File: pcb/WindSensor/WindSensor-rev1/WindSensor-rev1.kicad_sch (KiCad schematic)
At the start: 14 parts, among them U1 Sensor_Wind, U2 Sensor_Wind, U3 Sensor_Wind, U4 LP5814DRLR

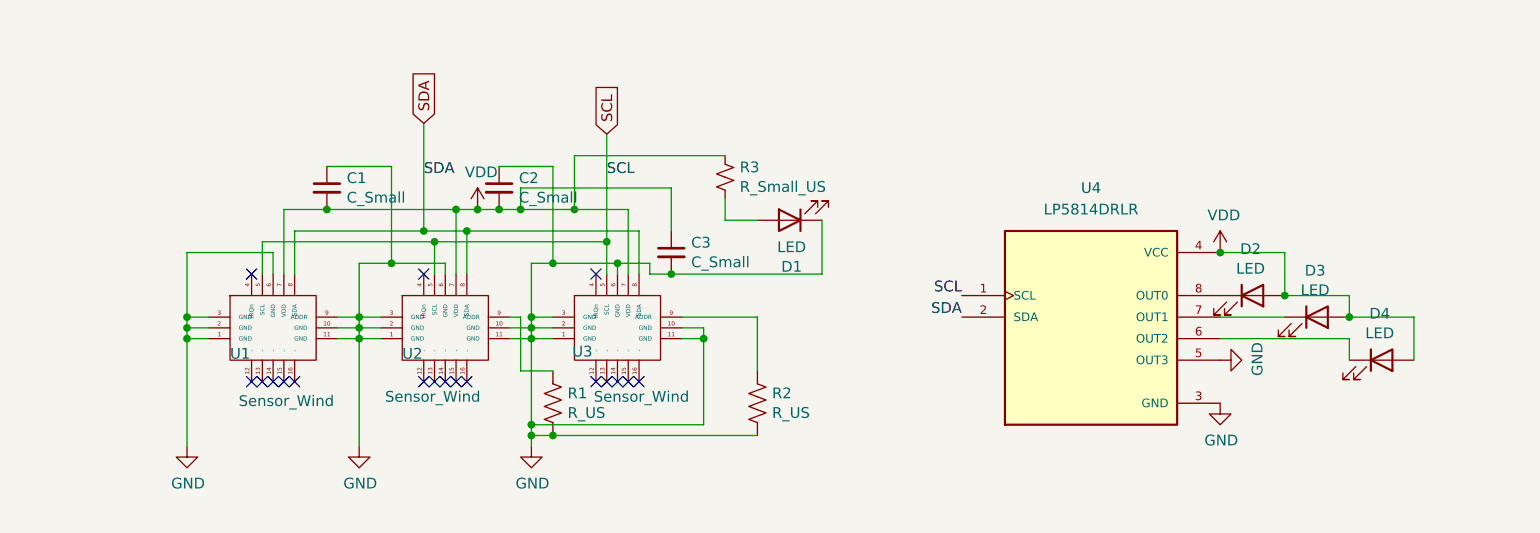
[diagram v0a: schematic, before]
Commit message: getting there
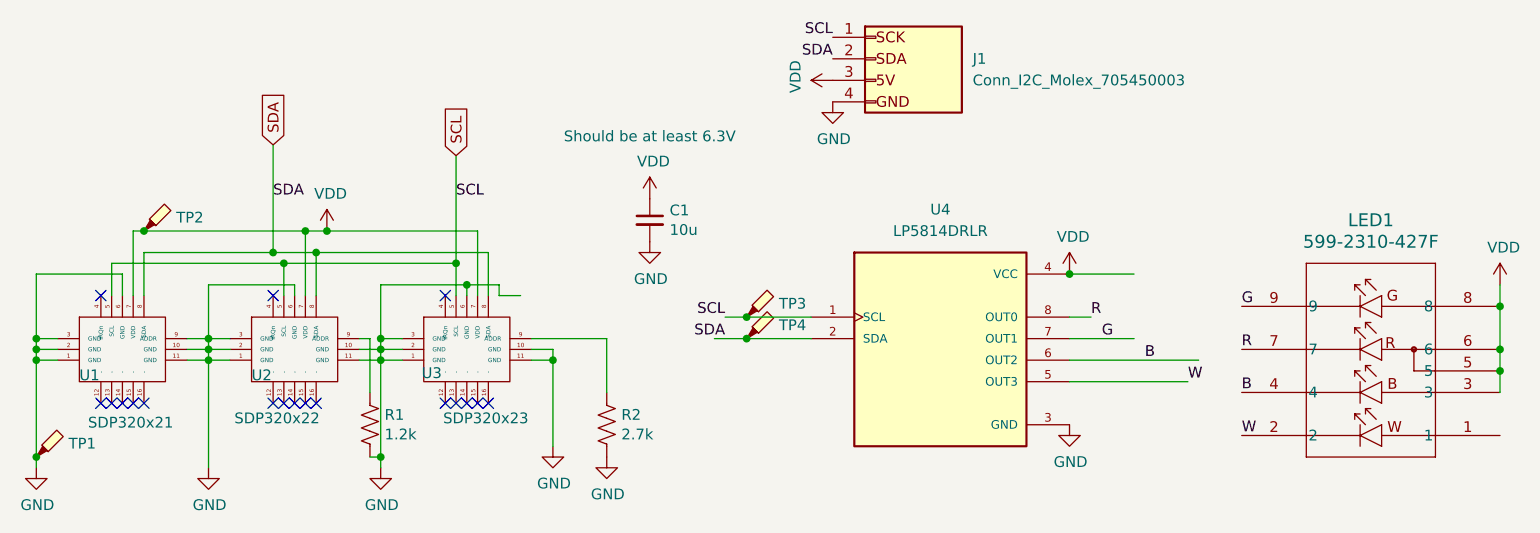
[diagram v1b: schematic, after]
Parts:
- removed C2, C3: C_Small, Capacitor_SMD:C_0201_0603Metric, symbol Device:C_Small
- removed D1, D2, D3, D4: LED, WindSensor:LED_3528, symbol Device:LED
- removed R3: R_Small_US, Resistor_SMD:R_0201_0603Metric, symbol Device:R_Small_US
- added J1: Conn_I2C_Molex_705450003, WindSensor:CONN_SD-74099-1000_04_MOL, symbol WindSensor:Conn_I2C_Molex_740990604
- added LED1: 599-2310-427F, WindSensor:599-2310_DIA, symbol WindSensor:599-2310-427F
- added TP1, TP2, TP3, TP4: TestPoint_Probe_autonamed, argo:TestPoint_scope_probe_autonamed, symbol argo:TestPoint_Probe_autonamed
- C1: value C_Small -> 10u; footprint Capacitor_SMD:C_0201_0603Metric -> Capacitor_SMD:C_0603_1608Metric_Pad1.08x0.95mm_HandSolder
- R1: value R_US -> 1.2k; footprint Resistor_SMD:R_0201_0603Metric -> Resistor_SMD:R_0603_1608Metric_Pad0.98x0.95mm_HandSolder
- R2: value R_US -> 2.7k; footprint Resistor_SMD:R_0201_0603Metric -> Resistor_SMD:R_0603_1608Metric_Pad0.98x0.95mm_HandSolder
- U1: value Sensor_Wind -> SDP320x21
- U2: value Sensor_Wind -> SDP320x22
- U3: value Sensor_Wind -> SDP320x23
- U4: footprint LP5814DRLR:IC_LP5814DRLR -> WindSensor:IC_LP5814DRLR; Product page (none) -> https://www.ti.com/product/LP5814
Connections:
- net GND: now also C1.2, U1.17 (GND), U1.18 (GND), U2.17 (GND), U2.18 (GND), U3.17 (GND), U3.18 (GND), J1.4 (GND), TP1.1; no longer C1.1, U4.5 (OUT3)
- net SCL: now also J1.1 (SCLK), TP3.1
- net SDA: now also J1.2 (SDA), TP4.1
- net VDD: now also C1.1, J1.3 (5V), LED1.3, LED1.5, LED1.6, LED1.8, TP2.1; no longer C1.2
- net G: now reaches U4.7 (OUT1)
- net G: now also LED1.9
- net B: now reaches U4.6 (OUT2)
- net B: now also LED1.4
- net R: now reaches U4.8 (OUT0)
- net R: now also LED1.7
- new net W: LED1.2, U4.5 (OUT3)
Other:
- moved on the sheet: R1, R2, U1, U2, U3, U4
